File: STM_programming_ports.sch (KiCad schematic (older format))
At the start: 11 parts, among them J1 Conn_ARM_JTAG_SWD_10, J2 st-linkv2-clone-port, J3 Conn_ARM_JTAG_SWD_20, J4 Conn_01x02_Male, J5 6PinDebugPort, J6 FOUR_WIRE_CONN, J7 st-linkv2-clone-port, J8 SW_WITH_RST, SW1 SW_Push

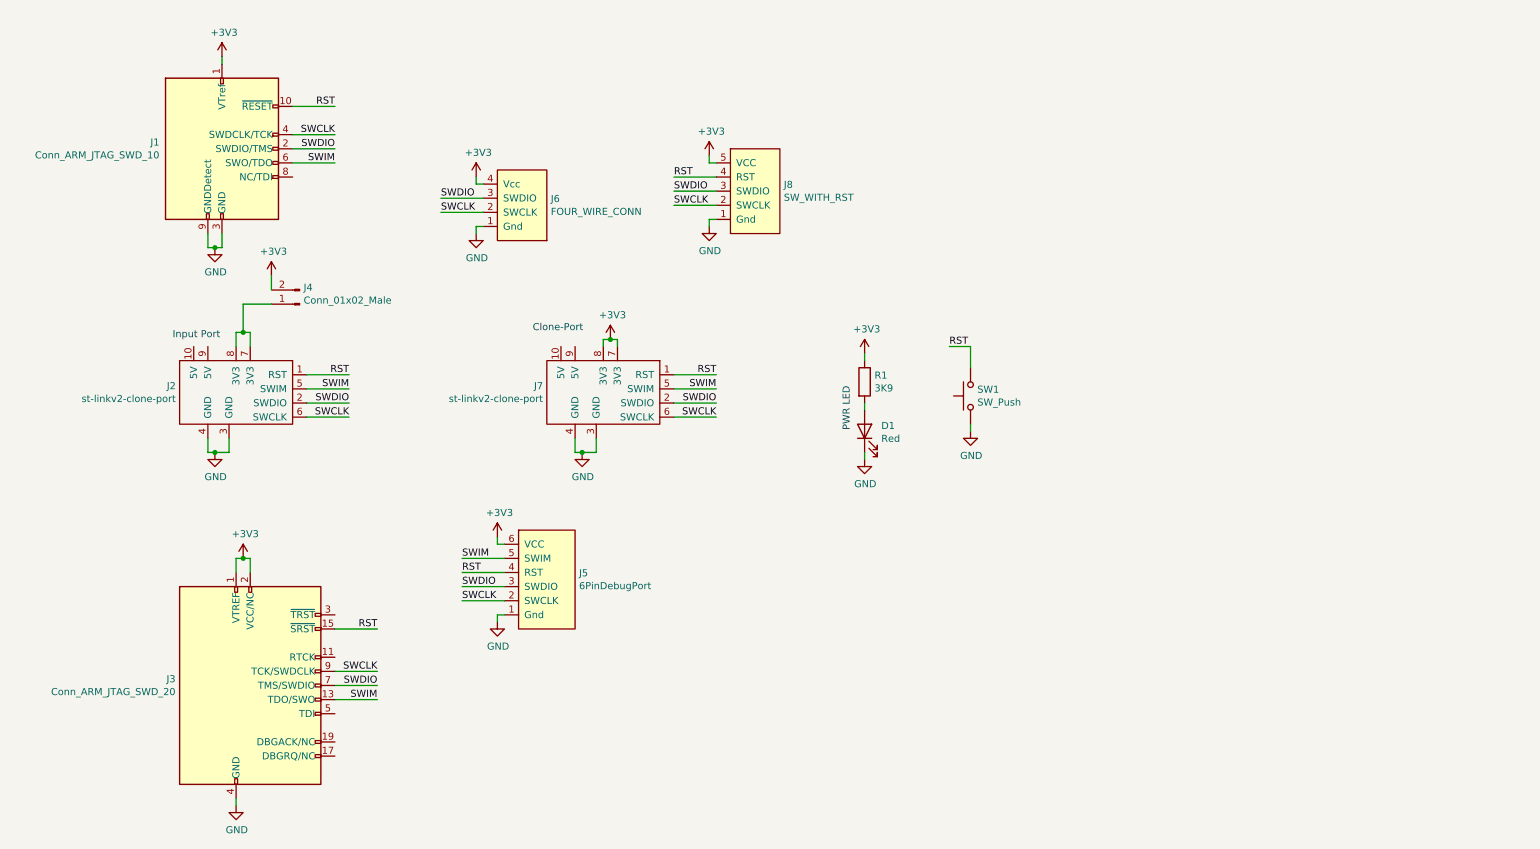
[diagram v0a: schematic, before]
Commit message: Written README
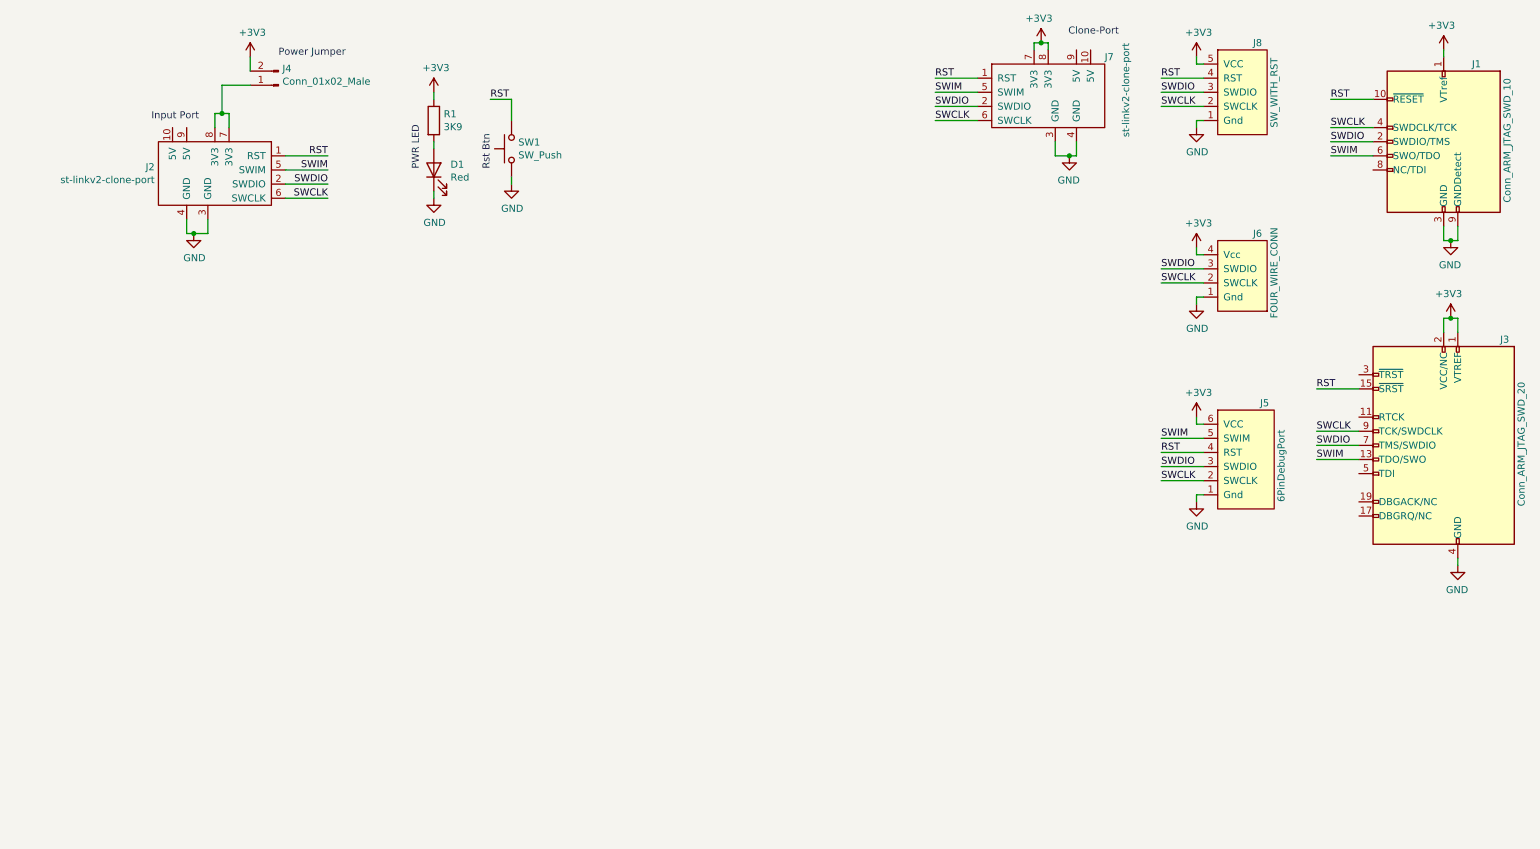
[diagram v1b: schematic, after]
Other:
- note added: "Power Jumper"
- note added: "Rst Btn"
- moved on the sheet: D1, J1, J2, J3, J4, J5, J6, J7, J8, R1, SW1
